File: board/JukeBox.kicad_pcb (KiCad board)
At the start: 2 copper layers, 90 x 90 mm, 73 parts, among them J1 USB4105-GF-A, J2 Conn_01x03, J3 Conn_01x04, J4 Conn_01x08, J5 Conn_01x01, J6 Conn_01x03, J7 Conn_01x03, J8 Conn_01x01, SW1 SW_SPST, SW10 SW_SPST, SW11 SW_SPST, SW12 SW_SPST, SW2 SW_SPST, SW3 SW_SPST, SW4 SW_SPST, SW5 SW_SPST, SW6 SW_SPST, SW7 SW_SPST, SW8 SW_SPST, SW9 SW_SPST, U1 NCP1117-3.3_SOT223, U2 W25Q128JVS, U3 RP2040, Y1 ABLS-12.000MHZ-B4-T

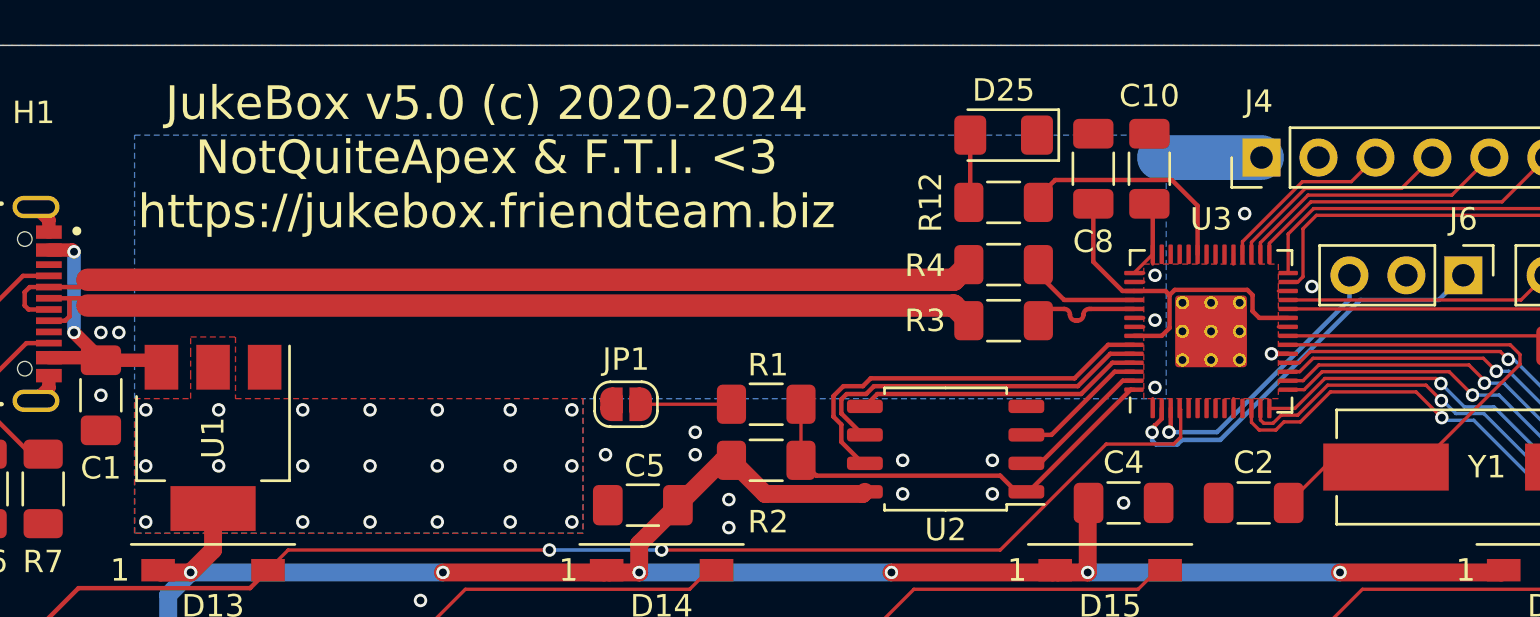
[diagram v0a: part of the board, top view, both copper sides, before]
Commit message: minor adjustments
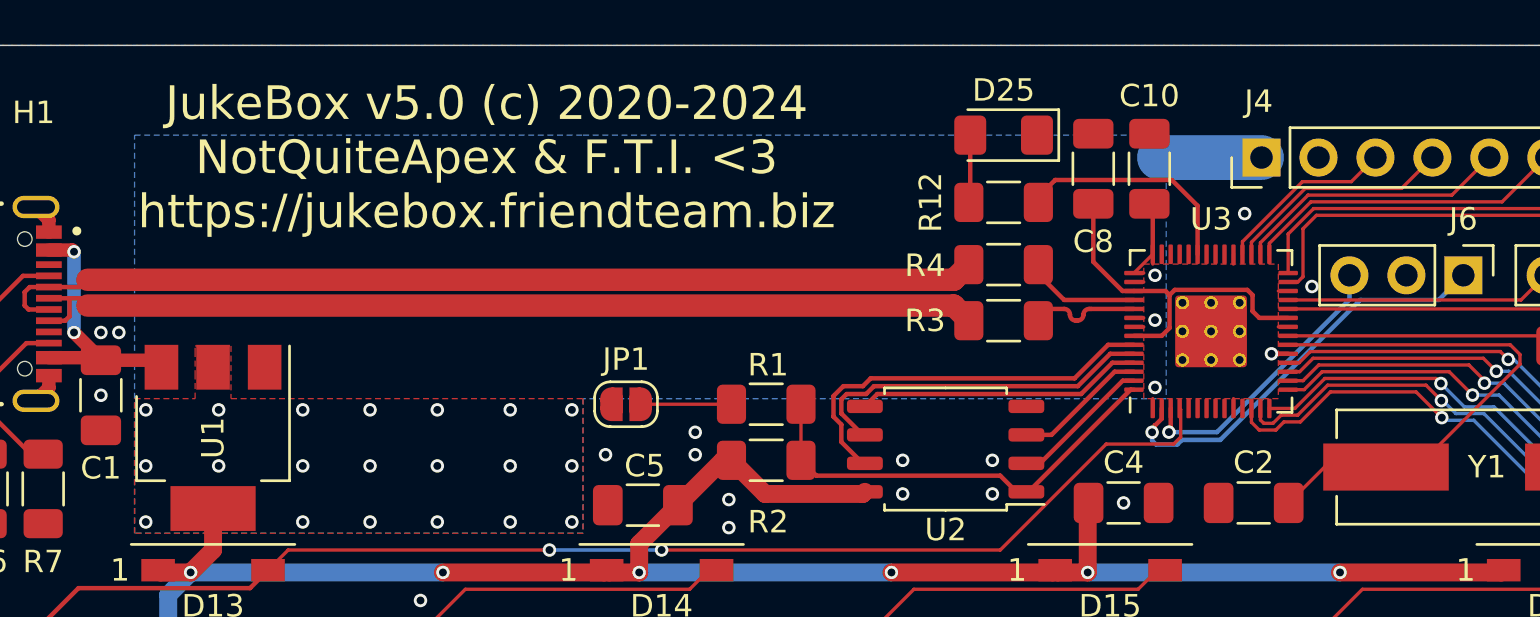
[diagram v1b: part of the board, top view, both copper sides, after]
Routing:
- net /XIN: track 24.6 -> 23.8 mm
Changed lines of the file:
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@@
       (viasonmask false)
       (mode 1)
-      (useauxorigin false)
+      (useauxorigin true)
       (hpglpennumber 1)
       (hpglpenspeed 20)
@@
     (fp_line (start -1.6 -0.4) (end -1.6 0.8) (layer "F.Fab") (width 0.1))
     (fp_line (start 1.6 0.8) (end 1.6 -0.8) (layer "F.Fab") (width 0.1))
-    (pad "1" smd roundrect (at -1.4875 0 180) (size 1.425 1.75) (layers "F.Cu" "F.Paste" "F.Mask") (roundrect_rratio 0.175439)
+    (pad "1" smd roundrect (at -1.4875 0 180) (size 1.425 1.75) (layers "F.Cu" "F.Paste" "F.Mask") (roundrect_rratio 0.1754392982)
       (net 1 "GND") (pinfunction "K") (pintype "passive"))
-    (pad "2" smd roundrect (at 1.4875 0 180) (size 1.425 1.75) (layers "F.Cu" "F.Paste" "F.Mask") (roundrect_rratio 0.175439)
+    (pad "2" smd roundrect (at 1.4875 0 180) (size 1.425 1.75) (layers "F.Cu" "F.Paste" "F.Mask") (roundrect_rratio 0.1754392982)
       (net 69 "Net-(D25-Pad2)") (pinfunction "A") (pintype "passive"))
     (model "${KICAD6_3DMODEL_DIR}/Diode_SMD.3dshapes/D_1206_3216Metric.wrl"
@@
     (fp_line (start 1.6 -0.8) (end 1.6 0.8) (layer "F.Fab") (width 0.1))
     (fp_line (start -1.6 -0.8) (end 1.6 -0.8) (layer "F.Fab") (width 0.1))
-    (pad "1" smd roundrect (at -1.55 0 180) (size 1.3 1.75) (layers "F.Cu" "F.Paste" "F.Mask") (roundrect_rratio 0.192308)
+    (pad "1" smd roundrect (at -1.55 0 180) (size 1.3 1.75) (layers "F.Cu" "F.Paste" "F.Mask") (roundrect_rratio 0.1923076923)
       (net 73 "/GPIO25") (pintype "passive"))
-    (pad "2" smd roundrect (at 1.55 0 180) (size 1.3 1.75) (layers "F.Cu" "F.Paste" "F.Mask") (roundrect_rratio 0.192308)
+    (pad "2" smd roundrect (at 1.55 0 180) (size 1.3 1.75) (layers "F.Cu" "F.Paste" "F.Mask") (roundrect_rratio 0.1923076923)
       (net 69 "Net-(D25-Pad2)") (pintype "passive"))
     (model "${KICAD6_3DMODEL_DIR}/Resistor_SMD.3dshapes/R_1206_3216Metric.wrl"
@@
   (via (at 176.39 67.8) (size 0.6) (drill 0.35) (layers "F.Cu" "B.Cu") (net 2))
   (segment (start 176.39 64.2) (end 176.39 67.8) (width 0.6) (layer "B.Cu") (net 2))
-  (segment (start 235.682463 74.4) (end 234.89 74.4) (width 0.15) (layer "F.Cu") (net 3))
   (segment (start 230.5275 68.35) (end 240.432463 68.35) (width 0.15) (layer "F.Cu") (net 3))
   (segment (start 232.1525 73.8) (end 230.5525 75.4) (width 0.15) (layer "F.Cu") (net 3))
@@
     (polygon
       (pts
-        (xy 183.59 70.75)
+        (xy 183.39 70.75)
         (xy 199.09 70.75)
         (xy 199.09 76.75)
         (xy 179.09 76.75)
         (xy 179.09 70.75)
-        (xy 181.59 70.75)
-        (xy 181.59 69.75)
-        (xy 181.59 68.75)
-        (xy 181.59 68)
-        (xy 183.59 68)
+        (xy 181.79 70.75)
+        (xy 181.79 69.75)
+        (xy 181.79 68.75)
+        (xy 181.79 68.4)
+        (xy 183.39 68.4)
       )
     )
